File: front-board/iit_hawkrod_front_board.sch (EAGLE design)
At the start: 31 parts

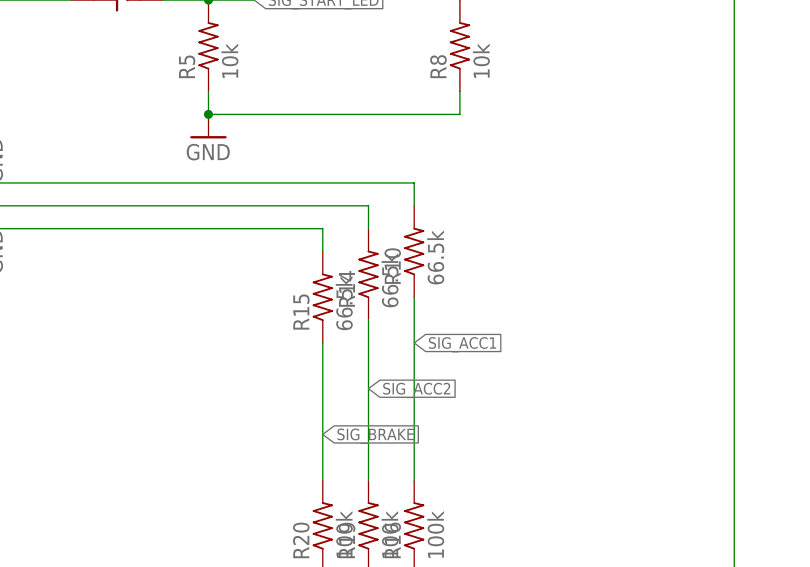
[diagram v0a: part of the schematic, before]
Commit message: Layout_Pre
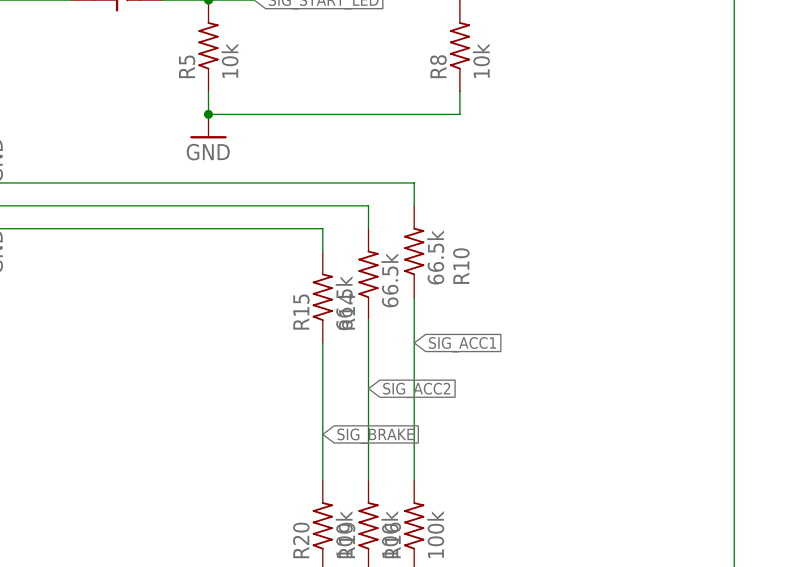
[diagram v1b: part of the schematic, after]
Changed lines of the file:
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@@
 </instance>
 <instance part="R10" gate="G$1" x="81.28" y="-33.02" smashed="yes" rot="R90">
-<attribute name="NAME" x="79.7814" y="-36.83" size="1.778" layer="95" rot="R90"/>
+<attribute name="NAME" x="87.4014" y="-36.83" size="1.778" layer="95" rot="R90"/>
 <attribute name="VALUE" x="84.582" y="-36.83" size="1.778" layer="96" rot="R90"/>
 </instance>
 <instance part="R14" gate="G$1" x="76.2" y="-35.56" smashed="yes" rot="R90">
-<attribute name="NAME" x="74.7014" y="-39.37" size="1.778" layer="95" rot="R90"/>
+<attribute name="NAME" x="74.7014" y="-41.91" size="1.778" layer="95" rot="R90"/>
 <attribute name="VALUE" x="79.502" y="-39.37" size="1.778" layer="96" rot="R90"/>
 </instance>
